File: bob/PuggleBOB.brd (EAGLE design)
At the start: 30.5 x 85.1 mm, 9 parts

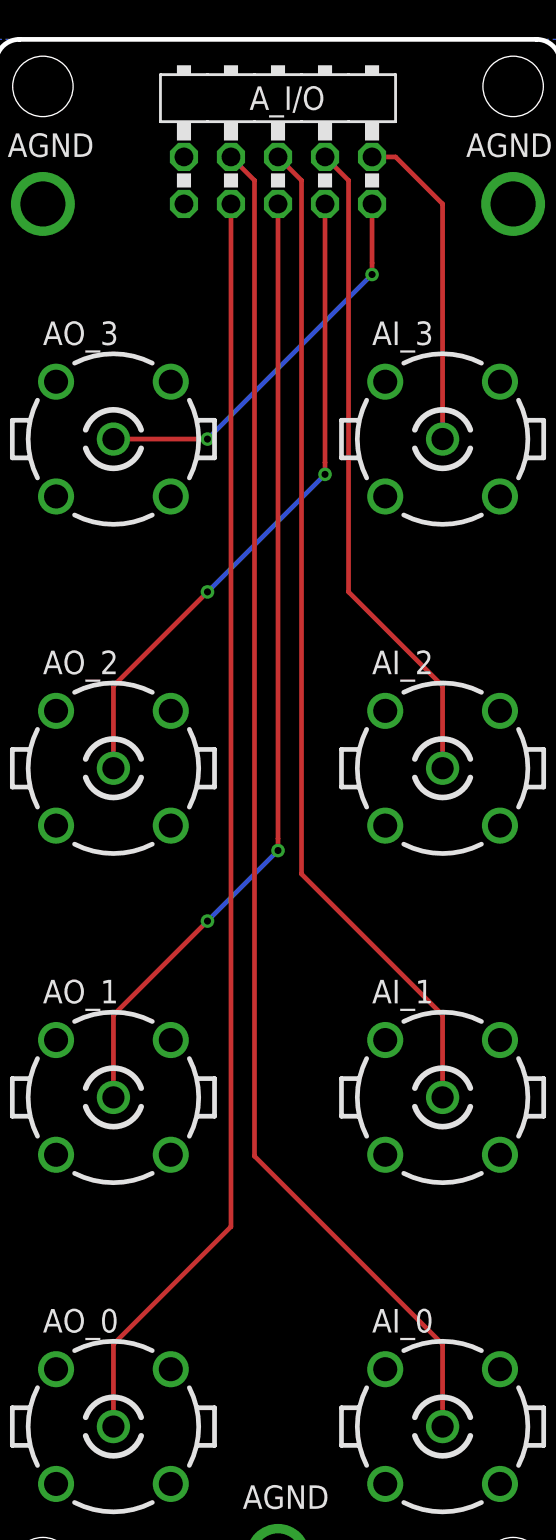
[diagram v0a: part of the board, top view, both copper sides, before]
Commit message: Finished BOB.
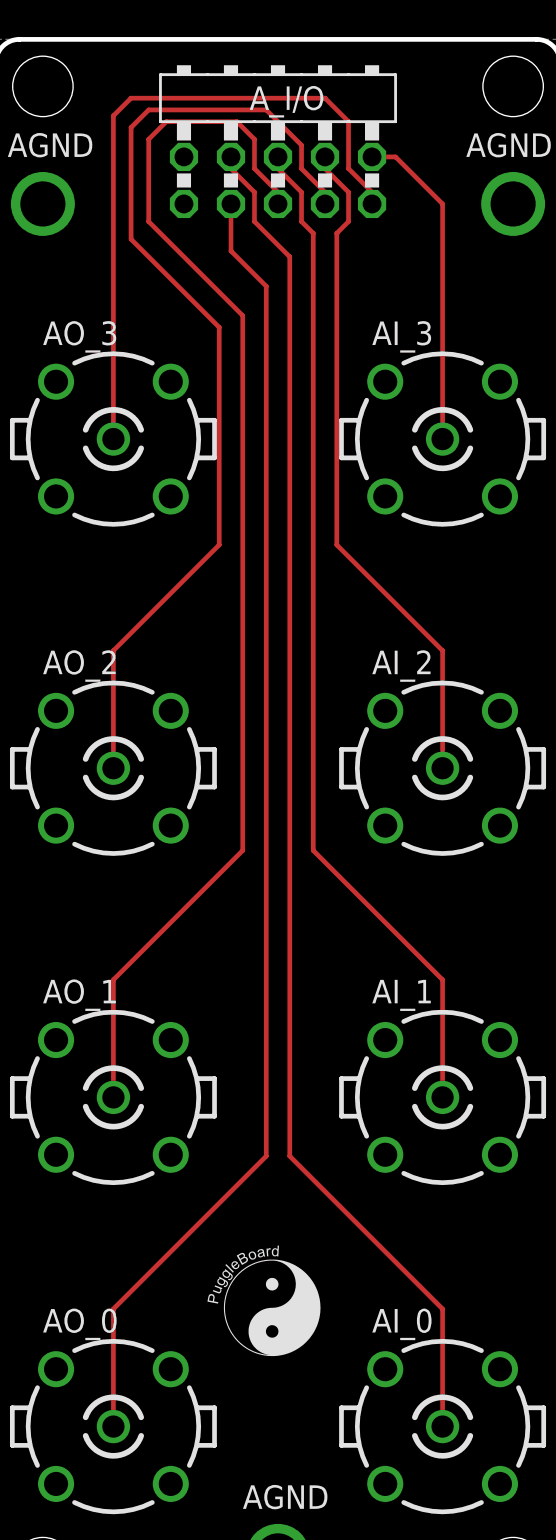
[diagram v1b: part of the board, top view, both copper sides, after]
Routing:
- net DAC_C: track 35.2 -> 53.0 mm, vias 2 -> 0
- net DAC_B: track 51.9 -> 67.3 mm, vias 2 -> 0
- net DAC_D: track 21.5 -> 36.1 mm, vias 2 -> 0
- net DAC_A: track 68.7 -> 70.2 mm
- net ADC_C: track 35.7 -> 36.2 mm

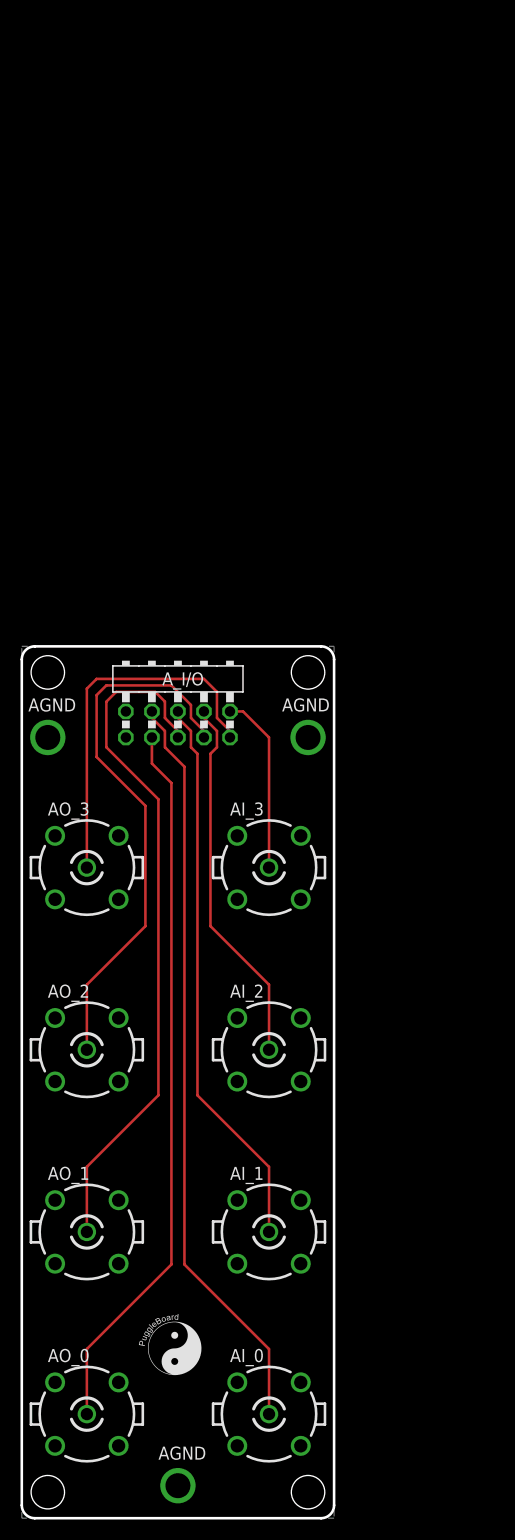
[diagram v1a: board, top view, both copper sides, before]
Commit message: Minor changes.
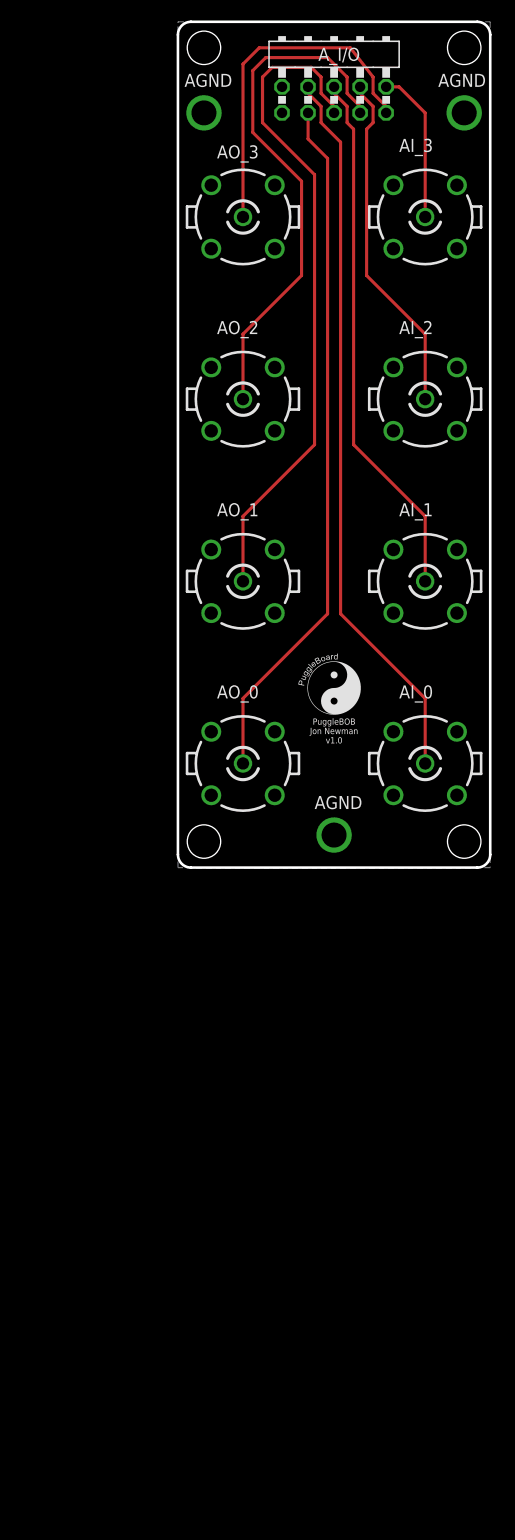
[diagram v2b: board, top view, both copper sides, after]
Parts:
- moved AI_0 65.3 mm to (24.1, 10.2)
- moved AI_1 65.3 mm to (24.1, 27.9)
- moved AI_2 65.3 mm to (24.1, 45.7)
- moved AI_3 65.3 mm to (24.1, 63.5)
- moved AO_0 65.3 mm to (6.35, 10.2)
- moved AO_1 65.3 mm to (6.35, 27.9)
- moved AO_2 65.3 mm to (6.35, 45.7)
- moved AO_3 65.3 mm to (6.35, 63.5)
- moved A_I/O 62.8 mm to (15.2, 78.7)
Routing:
- net ADC_A: track 73.3 -> 70.8 mm
- net DAC_A: track 70.2 -> 67.7 mm
- net ADC_D: track 17.6 -> 15.0 mm
- net ADC_B: track 54.5 -> 51.9 mm
- net DAC_B: track 67.3 -> 64.7 mm
- net ADC_C: track 36.2 -> 33.6 mm
- net DAC_D: track 36.1 -> 33.7 mm
- net DAC_C: track 53.0 -> 50.9 mm
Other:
- board size 30.5 x 85.1 mm -> 30.5 x 82.5 mm
- board text added: "PuggleBOB Jon Newman v1.0"
